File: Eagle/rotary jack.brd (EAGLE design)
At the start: 49.2 x 21.6 mm, 11 parts

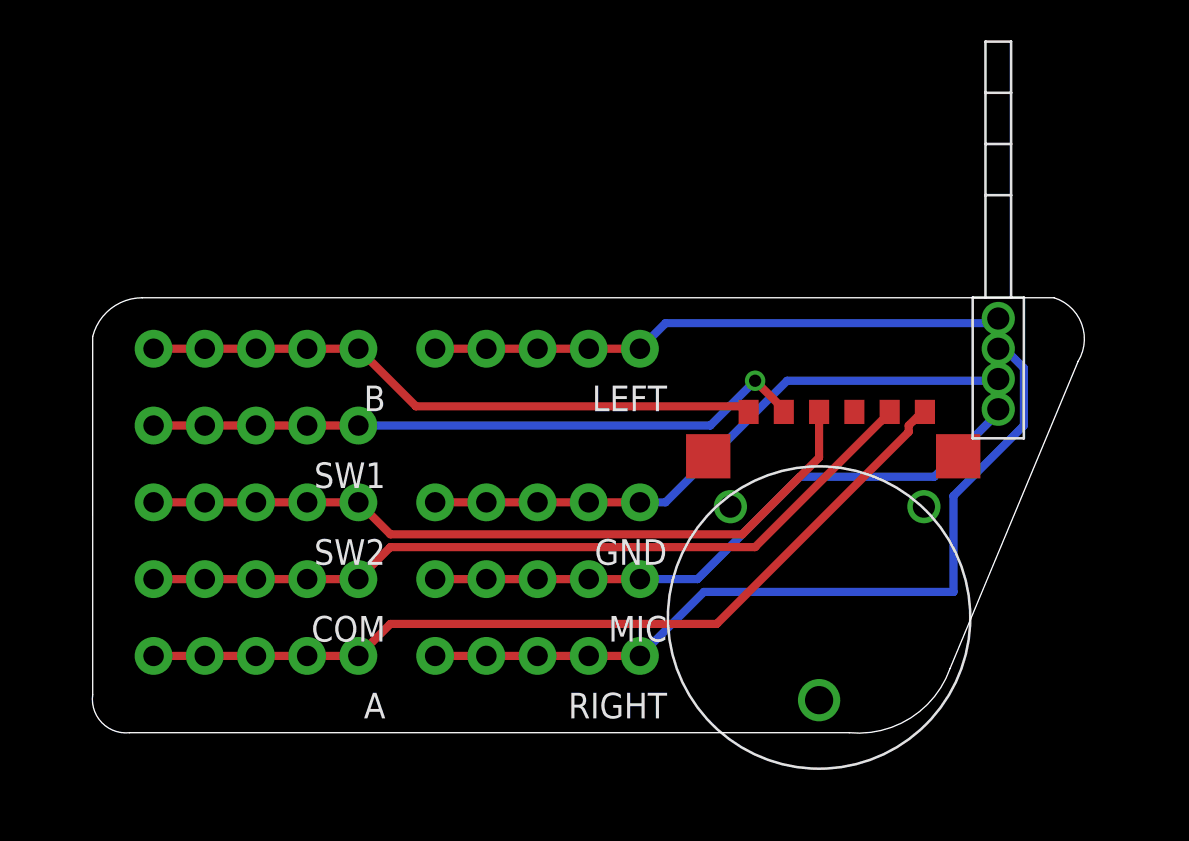
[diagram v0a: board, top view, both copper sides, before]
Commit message: dev
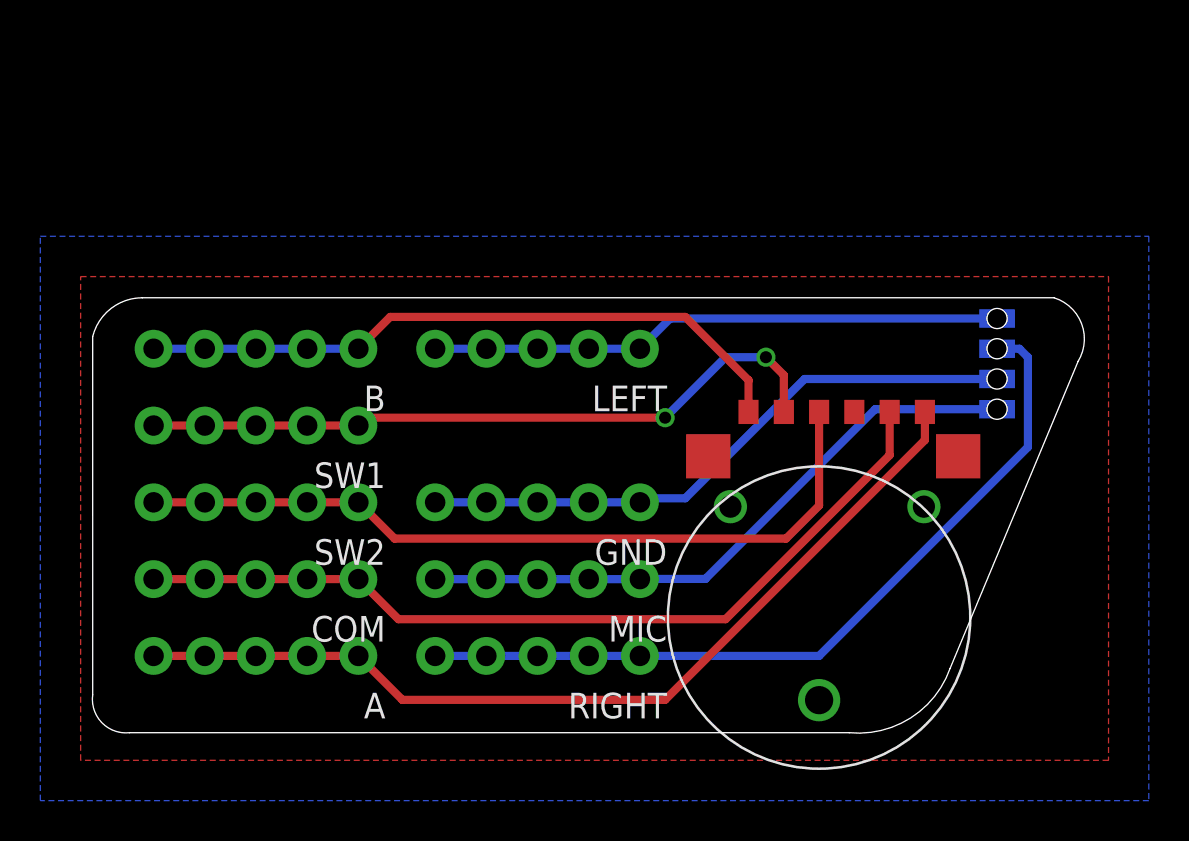
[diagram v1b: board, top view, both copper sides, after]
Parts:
- moved U$2 0.06 mm to (49.5, 58.4), flipped to the bottom
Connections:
- net N$3 renamed GND
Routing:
- net COM: track 40.0 -> 42.9 mm
- net A: track 43.5 -> 45.9 mm
- net B: track 30.8 -> 33.1 mm
- net SW1: track 32.9 -> 34.9 mm, vias 1 -> 2
- net SW2: track 37.5 -> 39.1 mm
- net N$2: track 41.3 -> 39.9 mm
- added copper zone on layer 1, net GND
- added copper zone on layer 16, net GND
